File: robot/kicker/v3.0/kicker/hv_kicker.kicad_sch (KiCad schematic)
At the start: 0 parts

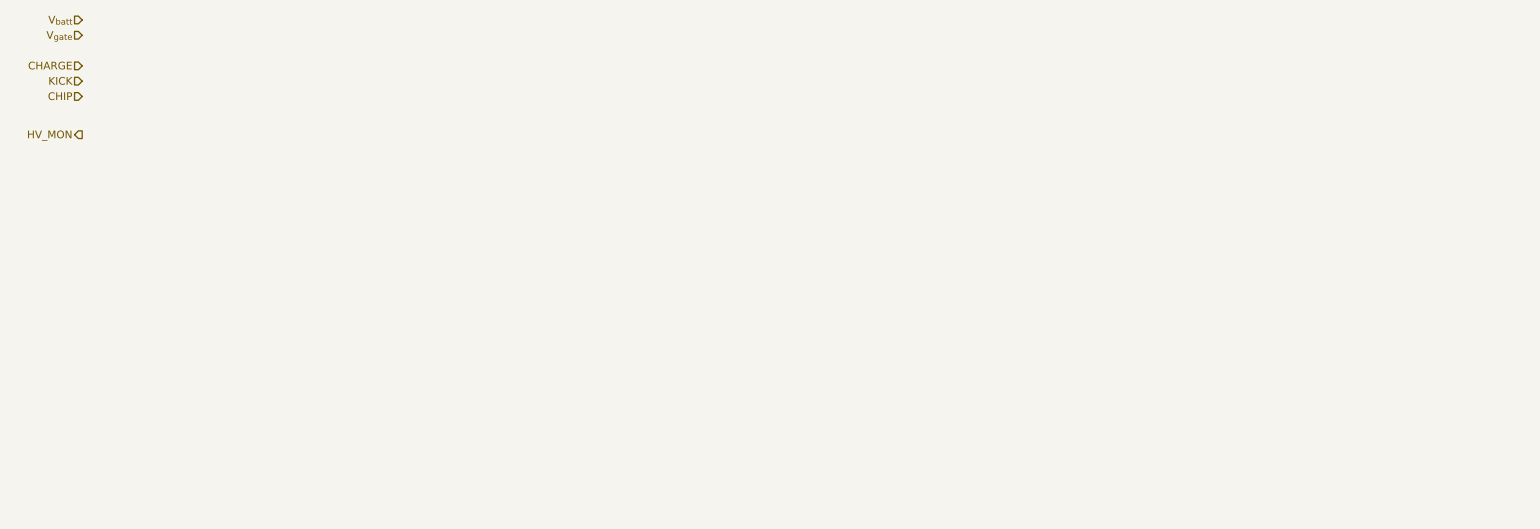
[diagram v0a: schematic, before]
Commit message: kicker work
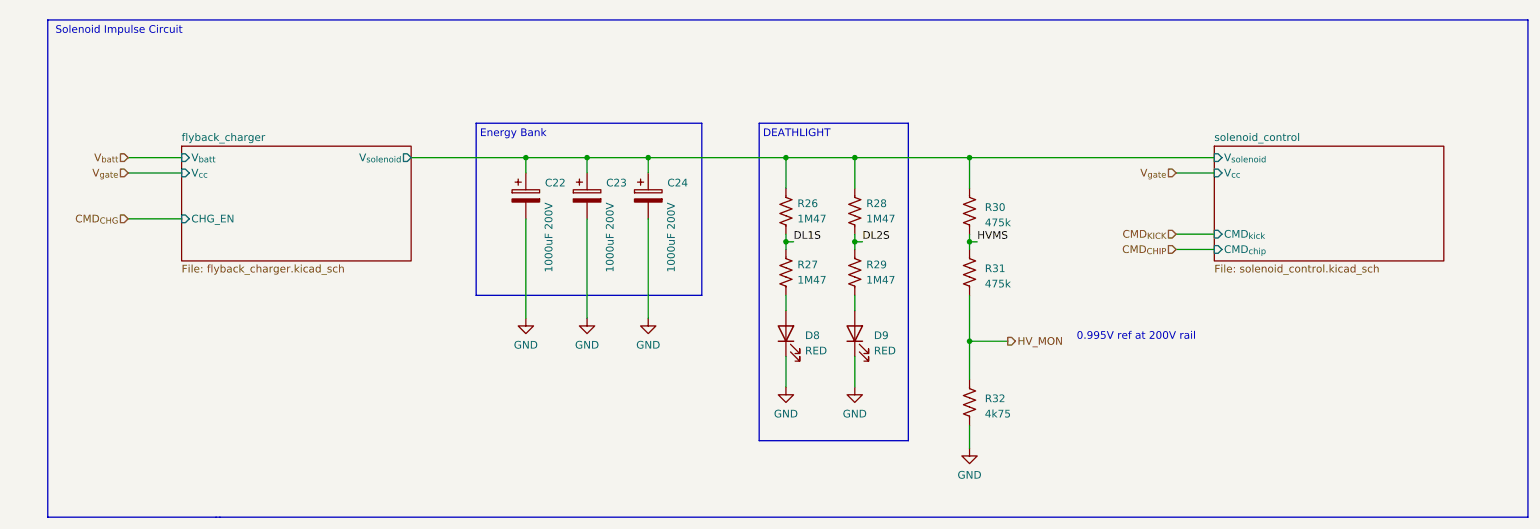
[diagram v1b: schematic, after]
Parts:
- added C22, C23, C24: 1000uF 200V, AT-Capacitors:ESMQ201VSN102MQ35S, symbol Device:C_Polarized
- added D8, D9: RED, AT-LED:LED0603, symbol Device:LED
- added R26, R27, R28, R29: 1M47, Resistor_SMD:R_0603_1608Metric, symbol Device:R_US
- added R30, R31: 475k, Resistor_SMD:R_0603_1608Metric, symbol Device:R_US
- added R32: 4k75, Resistor_SMD:R_0603_1608Metric, symbol Device:R_US
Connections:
- net HV_MON: now also R31.2, R32.1
- new net: D8.2 (A), R27.2
- new net: D9.2 (A), R29.2
- new net DL1S: R26.2, R27.1
- new net DL2S: R28.2, R29.1
- new net GND: C22.2, C23.2, C24.2, D8.1 (K), D9.1 (K), R32.2
- new net HVMS: R30.2, R31.1
- new net flyback_charger/V_{solenoid}: C22.1, C23.1, C24.1, R26.1, R28.1, R30.1
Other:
- added sheet flyback_charger (flyback_charger.kicad_sch)
- added sheet solenoid_control (solenoid_control.kicad_sch)
- note added: "0.995V ref at 200V rail"
- note added: "DEATHLIGHT"
- note added: "Energy Bank"
- note added: "Solenoid Impulse Circuit"
